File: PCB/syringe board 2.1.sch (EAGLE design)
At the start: 42 parts, among them IC1 A3967SLB, J1 RJ45, J2 AVR_SPI_PROG_3X2NS, Q1 RESONATOR_CSTCE_V, U1 ATMEGA328P_TQFP, U2 PCA9306

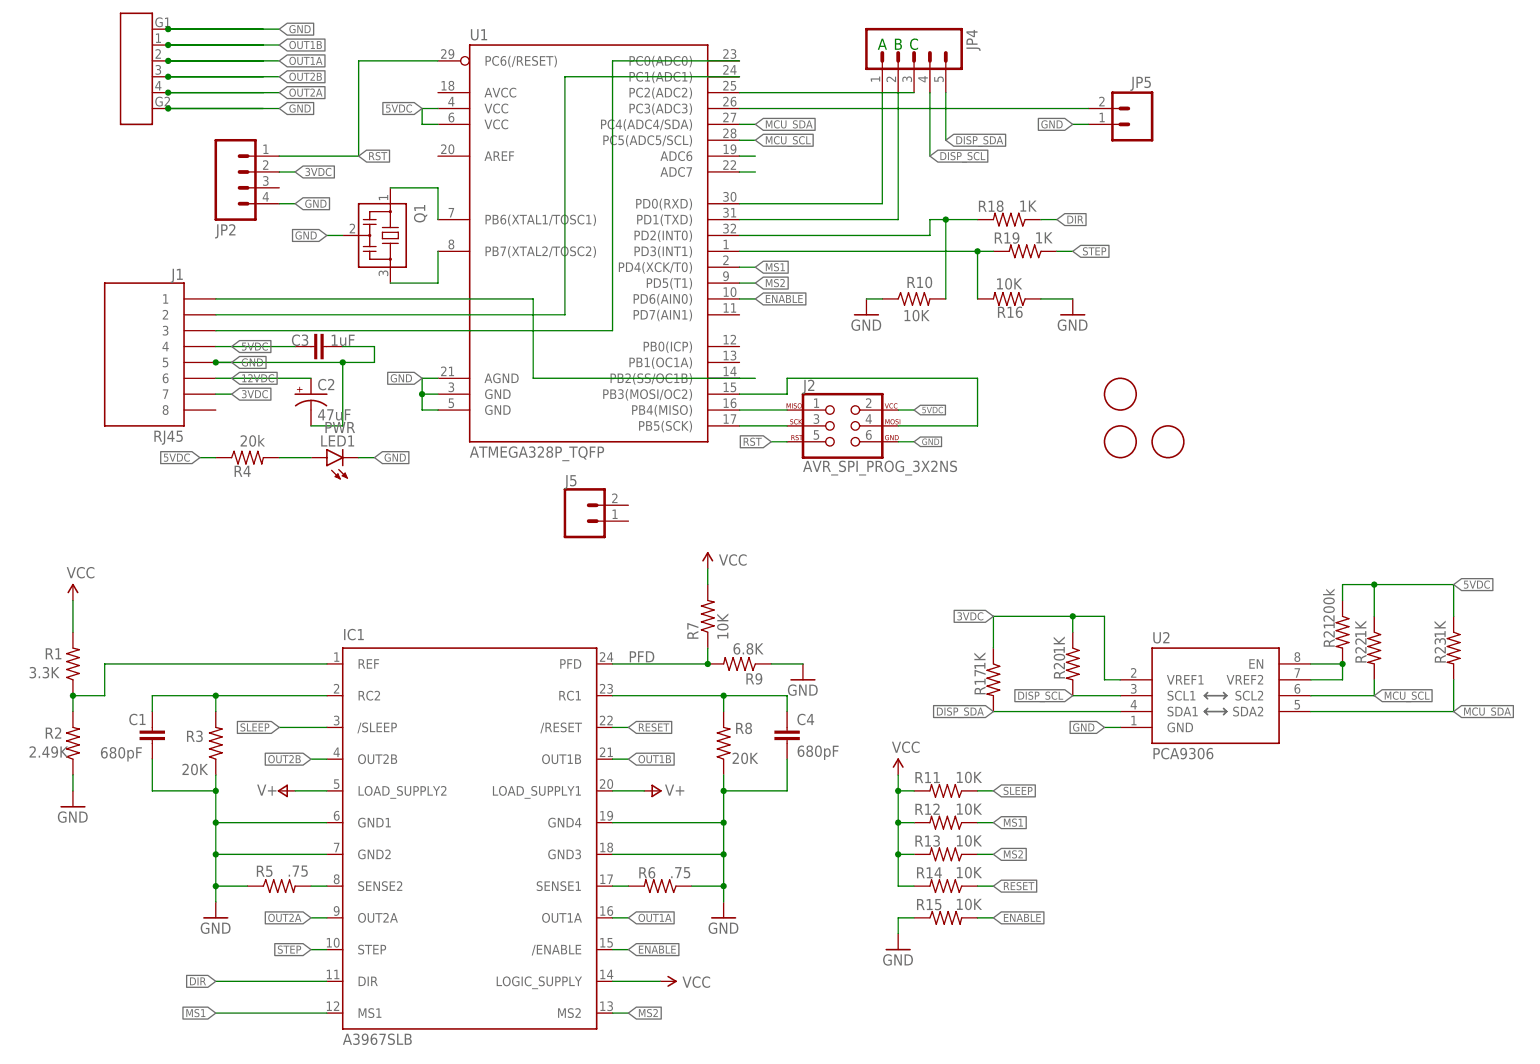
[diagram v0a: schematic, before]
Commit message: latest PCB
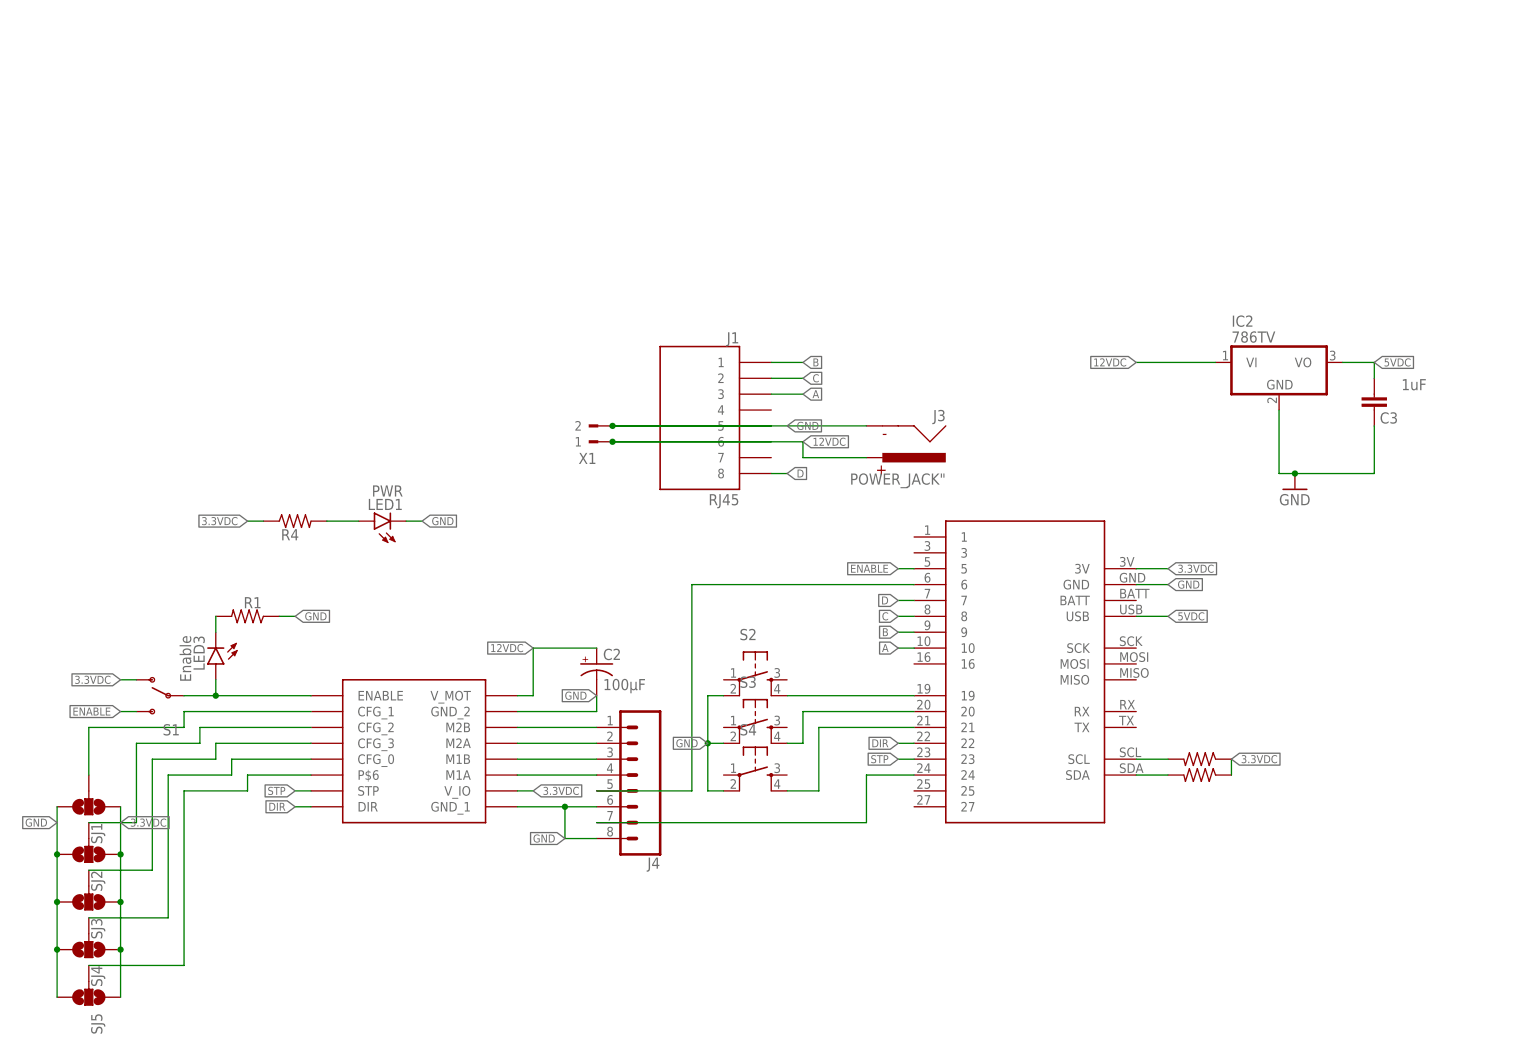
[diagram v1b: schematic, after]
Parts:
- removed C1, C4: 680pF, SparkFun-Capacitors:CAP0603-CAP
- removed IC1: A3967SLB, Allegro:A3967SLB
- removed J2: AVR_SPI_PROG_3X2NS, SparkFun-Connectors:AVR_SPI_PROG_3X2NS
- removed J5: (no value), SparkFun-Connectors:CONN_021X02_NO_SILK
- removed JP2: (no value), SparkFun-Connectors:M04NO_SILK_ALL_ROUND
- removed JP4: (no value), SparkFun-Connectors:M05NO_SILK
- removed JP5: (no value), SparkFun-Connectors:M021X02_NO_SILK
- removed Q1: RESONATOR_CSTCE_V, Andy-library:RESONATOR_CSTCE_V
- removed R10, R11, R12, R13, R14, R15, R16, R7: 10K, SparkFun-Resistors:RESISTOR0603
- removed R18, R19, R22, R23: 1K, SparkFun-Resistors:RESISTOR0603
- removed R2: 2.49K, SparkFun-Resistors:RESISTOR0603
- removed R21: 200k, SparkFun-Resistors:RESISTOR0603
- removed R3, R8: 20K, SparkFun-Resistors:RESISTOR0603
- removed R5, R6: .75, SparkFun-Resistors:RESISTOR0805-RES
- removed R9: 6.8K, SparkFun-Resistors:RESISTOR0603
- removed U$3: FIDUCIAL, adafruit:FIDUCIAL
- removed U$5: OMRON_4PIN, Andy-library:OMRON_4PIN
- removed U1: ATMEGA328P_TQFP, SparkFun-DigitalIC:ATMEGA328P_TQFP
- removed U2: PCA9306, SparkFun-DigitalIC:PCA9306
- added IC2: 786TV, Andy-library:786TV
- added J3: POWER_JACK", Andy-library:POWER_JACK"
- added J4: (no value), SparkFun-Connectors:CONN_08NO_SILK_FEMALE_PTH
- added LED3: Enable, Andy-library:LED0603
- added S1: (no value), Andy-library:SWITCH-SPDTVERTICAL_TOGGLE
- added S2, S3, S4: TAC_SWITCHSMD, Andy-library:TAC_SWITCHPTH
- added SJ1, SJ2, SJ3, SJ4, SJ5: (no value), SparkFun-Retired:SOLDERJUMPER_2WAYS
- added X1: (no value), con-weidmueller-sl35:90-2
- C2: value 47uF -> 100µF
- R1: value 3.3K -> (none)
- R17, R20: value 1K -> (none)
- R4: value 20k -> (none)
- U$1: value FIDUCIAL -> SILENT_STEP_STICK; device adafruit:FIDUCIAL -> Andy-library:SILENT_STEP_STICK
- U$2: value FIDUCIAL -> FEATHERFEAT; device adafruit:FIDUCIAL -> Andy-library:FEATHERFEAT
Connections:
- removed net 3VDC: J1.7, JP2.2, R17.1, R20.1, U2.VREF1
- removed net DIR_IN: R10.2, R18.2, U1.PD2(INT0)
- removed net DISP_SCL: JP4.4, R20.2, U2.SCL1
- removed net DISP_SDA: JP4.5, R17.2, U2.SDA1
- removed net MCU_SCL: R22.2, U1.PC5(ADC5/SCL), U2.SCL2
- removed net MCU_SDA: R23.2, U1.PC4(ADC4/SDA), U2.SDA2
- removed net MS1: IC1.MS1, R12.1, U1.PD4(XCK/T0)
- removed net MS2: IC1.MS2, R13.1, U1.PD5(T1)
- removed net N$17: JP4.3, U1.PC2(ADC2)
- removed net N$18: U1.ADC6
- removed net N$19: JP5.2, U1.PC3(ADC3)
- removed net N$20: J1.2, U1.PC1(ADC1)
- removed net N$21: J1.1, U1.PB2(SS/OC1B)
- removed net N$5: C1.1, IC1.RC2, R3.2
- removed net OUT1A: IC1.OUT1A, U$5.P$2
- removed net OUT1B: IC1.OUT1B, U$5.P$1
- removed net OUT2A: IC1.OUT2A, U$5.P$4
- removed net OUT2B: IC1.OUT2B, U$5.P$3
- removed net PFD: IC1.PFD, R7.1, R9.2
- removed net RESET: IC1./RESET, R14.1
- removed net RST: J2.5, JP2.1, U1.PC6(/RESET)
- removed net SLEEP: IC1./SLEEP, R11.1
- removed net STEP: IC1.STEP, R19.1
- removed net STEP_IN: R16.2, R19.2, U1.PD3(INT1)
- removed net VREF: IC1.REF, R1.1, R2.2
- new net 3.3VDC: R17.1, R20.1, R4.1, S1.O, SJ1.1, SJ2.1, SJ3.1, SJ4.1, SJ5.1, U$1.V_IO, U$2.3V
- new net A: J1.3, U$2.10
- new net B: J1.1, U$2.9
- new net C: J1.2, U$2.8
- new net CFG_0: SJ4.2, U$1.CFG_0
- new net CFG_1: SJ1.2, U$1.CFG_1
- new net CFG_2: SJ2.2, U$1.CFG_2
- new net CFG_3: SJ3.2, U$1.CFG_3
- new net D: J1.8, U$2.7
- new net N/C: SJ5.2, U$1.P$6
- new net STP: U$1.STP, U$2.23
- net 12VDC: now also IC2.VI, J3.PWR, U$1.V_MOT, X1.1; no longer IC1.LOAD_SUPPLY1, IC1.LOAD_SUPPLY2
- net 5VDC: now also C3.2, IC2.VO, U$2.USB; no longer C3.1, IC1.LOGIC_SUPPLY, J1.4, J2.2, R1.2, R11.2, R12.2, R13.2, R14.2, R21.1, R22.1, R23.1, R4.1, R7.2, U1.VCC@4, U1.VCC@6
- net DIR: now also U$1.DIR, U$2.22; no longer IC1.DIR, R18.1
- net ENABLE: now also S1.S, U$2.5; no longer IC1./ENABLE, R15.2, U1.PD6(AIN0)
- net GND: now also C3.1, IC2.GND, J3.GND, J4.6, J4.8, R1.1, S2.2, S3.2, S4.2, SJ1.3, SJ2.3, SJ3.3, SJ4.3, SJ5.3, U$1.GND_1, U$1.GND_2, U$2.GND, X1.2; no longer C1.2, C3.2, C4.2, IC1.GND1, IC1.GND2, IC1.GND3, IC1.GND4, J2.6, JP2.4, JP5.1, Q1.2, R10.1, R15.1, R16.1, R2.1, R3.1, R5.1, R6.1, R8.1, R9.1, U$5.GND1, U$5.GND2, U1.AGND, U1.GND@3, U1.GND@5, U2.GND
- net N$1: now also R17.2, U$2.SCL; no longer IC1.SENSE2, R5.2
- net N$10: now also LED3.C, R1.2; no longer J2.3, U1.PB5(SCK)
- net N$11: now also S3.4, U$2.20; no longer J2.4, U1.PB3(MOSI/OC2)
- net N$12: now also S4.4, U$2.21; no longer J1.3, U1.PC0(ADC0)
- net N$14: now also J4.3, U$1.M1B; no longer U1.ADC7
- net N$15: now also J4.4, U$1.M1A; no longer JP4.1, U1.PD0(RXD)
- net N$16: now also J4.7, U$2.24; no longer JP4.2, U1.PD1(TXD)
- net N$2: now also J4.5, U$2.6; no longer Q1.1, U1.PB6(XTAL1/TOSC1)
- net N$3: now also R20.2, U$2.SDA; no longer IC1.SENSE1, R6.2
- net N$4: now also J4.1, U$1.M2B; no longer Q1.3, U1.PB7(XTAL2/TOSC2)
- net N$6: now also LED3.A, S1.P, U$1.ENABLE; no longer R21.2, U2.EN, U2.VREF2
- net N$7: now also S2.4, U$2.19; no longer C4.1, IC1.RC1, R8.2
- net N$9: now also J4.2, U$1.M2A; no longer J2.1, U1.PB4(MISO)
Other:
- note removed: "A"
- note removed: "B"
- note removed: "C"
- note removed: "Max Coil Current(in Amps) = Vref(in Volts)/6"
- note removed: "Maximum current gives highest torque"
- note removed: "Minimum current gives smoothest microsteps"
- note removed: "PFD intermediate voltage"
- note removed: "Set for 'mixed-decay' mode."
- note removed: "Valid range 1.0V to Vcc"
- moved on the sheet: C2, C3, J1, LED1, R1, R4
